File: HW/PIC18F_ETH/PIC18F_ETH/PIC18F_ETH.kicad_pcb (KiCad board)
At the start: 2 copper layers, 160 x 80 mm, 136 parts, among them J2001 Conn_01x06, J4001 JST,2.54, J4002 JST,2.54, J4003 JST,2.54, J4004 JST,2.54, J4005 JST,2.54, J4006 JST,2.54, J4007 JST,2.54, J4008 JST,2.54, J4009 JST,2.54, J4010 JST,2.54, J4011 JST,2.54, J4012 JST,2.54, J4013 JST,2.54, J4014 JST,2.54, J4015 JST,2.54, J4016 JST,2.54, J4017 JST,2.54, J4018 JST,2.54, J4019 JST,2.54, J4020 JST,2.54, J4021 JST,2.54, J4022 JST,2.54, J4023 JST,2.54, J4024 JST,2.54, J4025 JST,2.54, J4026 JST,2.54, J5001 RJ45_LED_ETH_Shielded, U2001 PIC18F67J60T-I, U2002 25Mhz,50ppm, U2003 93AA46BT-I/OT, U4001 TLP241B, U4002 TLP241B, U4003 TLP241B, U4004 TLP241B, U4005 TLP241B, U4006 TLP241B, U4007 TLP241B, U4008 TLP241B, U6001 MCP2515T-E/ML, U6002 25Mhz,50ppm, U6003 ATA6561-GAQW

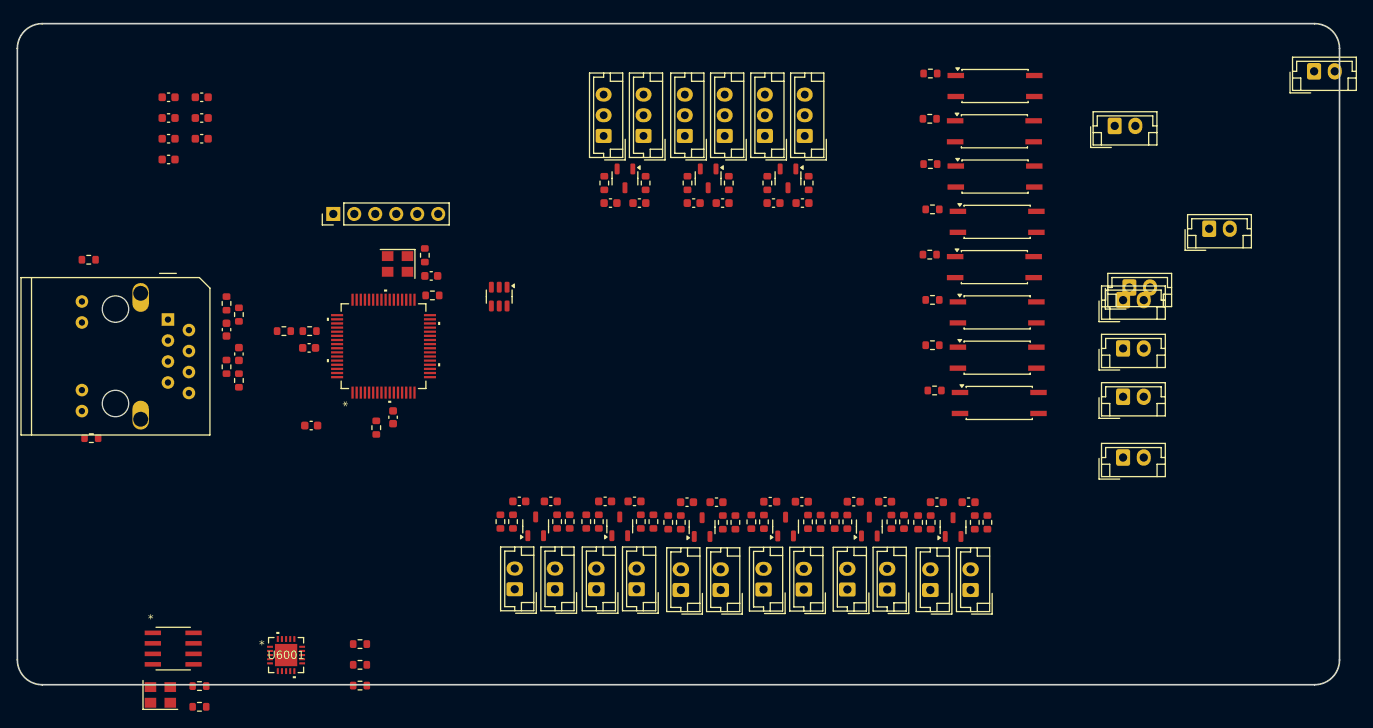
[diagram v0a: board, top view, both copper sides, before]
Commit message: .
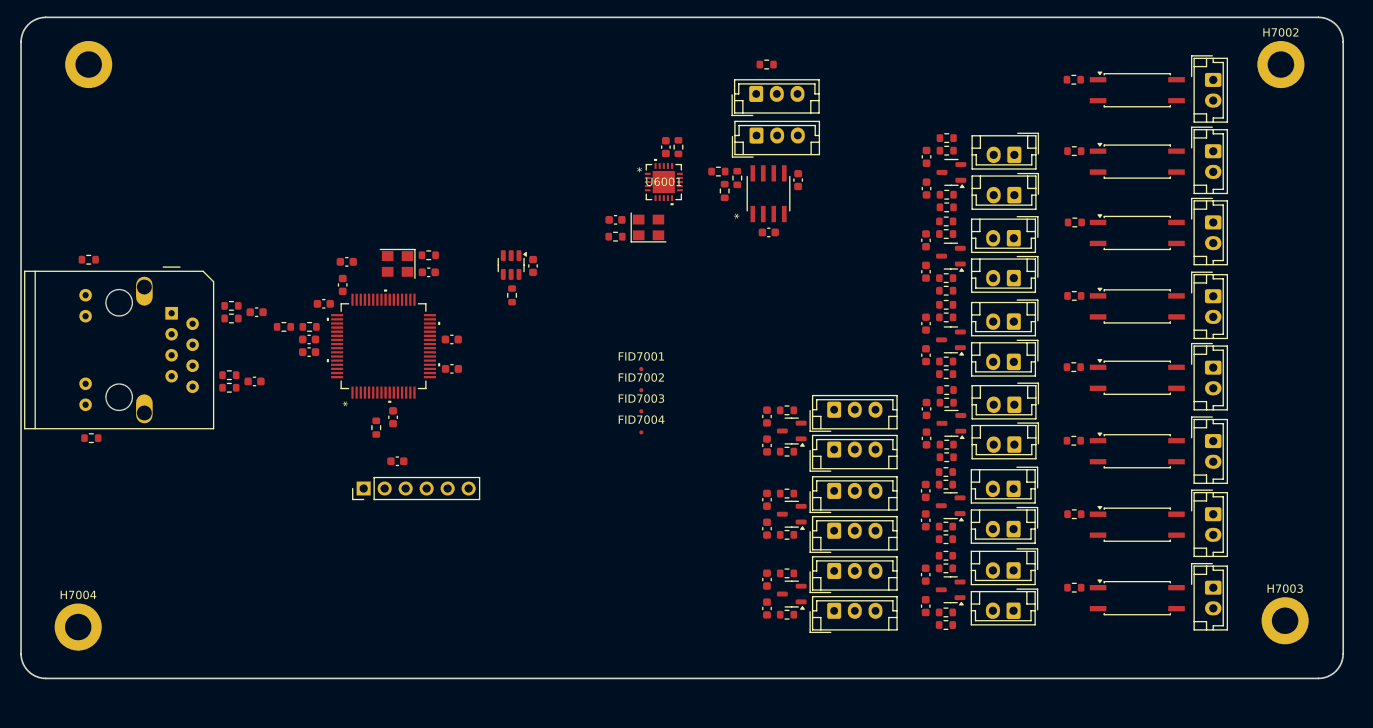
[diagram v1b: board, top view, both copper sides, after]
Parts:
- added C6001: 100n 25V, Capacitor_SMD:C_0603_1608Metric, F.Cu at (116.1, 124.7)
- added C6002: 100n 25V, Capacitor_SMD:C_0603_1608Metric, F.Cu at (122.2, 115.9)
- added C6003: 100n 25V, Capacitor_SMD:C_0603_1608Metric, F.Cu at (138.2, 119.9)
- added C6004: 100n 25V, Capacitor_SMD:C_0603_1608Metric, F.Cu at (134.6, 126.2)
- added FID7001: Fiducial_05_1, Fiducial:Fiducial_0.5mm_Mask1mm, F.Cu at (119.2, 142.8)
- added FID7002: Fiducial_05_1, Fiducial:Fiducial_0.5mm_Mask1mm, F.Cu at (119.2, 145.3)
- added FID7003: Fiducial_05_1, Fiducial:Fiducial_0.5mm_Mask1mm, F.Cu at (119.2, 147.9)
- added FID7004: Fiducial_05_1, Fiducial:Fiducial_0.5mm_Mask1mm, F.Cu at (119.2, 150.4)
- added H7001: MountingHole_Pad, MountingHole:MountingHole_3.2mm_M3_ISO7380_Pad, F.Cu at (52.3, 105.9)
- added H7002: MountingHole_Pad, MountingHole:MountingHole_3.2mm_M3_ISO7380_Pad, F.Cu at (196.6, 105.9)
- added H7003: MountingHole_Pad, MountingHole:MountingHole_3.2mm_M3_ISO7380_Pad, F.Cu at (197.1, 173.2)
- added H7004: MountingHole_Pad, MountingHole:MountingHole_3.2mm_M3_ISO7380_Pad, F.Cu at (51.1, 174.0)
- added J6001: JST,2.54, Connector_JST:JST_EH_B3B-EH-A_1x03_P2.50mm_Vertical, F.Cu at (133.1, 109.5)
- added J6002: JST,2.54, Connector_JST:JST_EH_B3B-EH-A_1x03_P2.50mm_Vertical, F.Cu at (133.1, 114.5)
- added R6006: 120R, Resistor_SMD:R_0603_1608Metric, F.Cu at (134.4, 105.9)
- moved U6003 90.7 mm to (134.6, 121.5), turned to 90 degrees
- moved R6002 89.1 mm to (123.7, 115.9), turned to -90 degrees
- moved U6002 81.8 mm to (120.1, 125.6)
- moved R6005 75.8 mm to (128.5, 118.9)
- moved R6004 74.5 mm to (130.8, 119.7), turned to 90 degrees
- moved R6001 74.1 mm to (116.1, 126.7)
- moved U6001 73.3 mm to (121.9, 120.1)
- moved R6003 70.4 mm to (129.3, 121.2), turned to -90 degrees
- moved J4011 60.4 mm to (164.2, 172.0), turned to 180 degrees
- moved J4006 57.6 mm to (142.5, 172.0), turned to 0 degrees
- moved J4012 55.5 mm to (164.2, 167.1), turned to 180 degrees
- moved R4007 55.3 mm to (156.1, 173.7), turned to 0 degrees
- moved R4034 53.5 mm to (156.1, 172.2), turned to 0 degrees
- moved J4005 53.3 mm to (142.5, 167.2), turned to 0 degrees
- moved J4018 52.9 mm to (164.3, 116.8), turned to 180 degrees
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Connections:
- net Net-(U6001-*RESET) renamed /CAN/CAN_CTRL_RST#
- U2001 pad 46: /ETH_Connector/ETH.RX+ -> /ETH_Connector/ETH.RX-
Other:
- copper layers 2 -> 4
